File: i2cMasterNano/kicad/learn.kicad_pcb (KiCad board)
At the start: 2 copper layers, 27 parts, among them J1 Conn_01x04_Male, J10 Conn_01x01, J2 Conn_01x04_Male, J3 Conn_01x04_Male, J4 Conn_01x04_Male, J5 Conn_01x04_Male, J6 Conn_01x04_Male, J7 Conn_01x04_Male, J8 Conn_01x04_Male, J9 Conn_01x01, SW1 SW_DIP_x03, U1 LM7805_TO220, U2 Arduino_Nano_R3

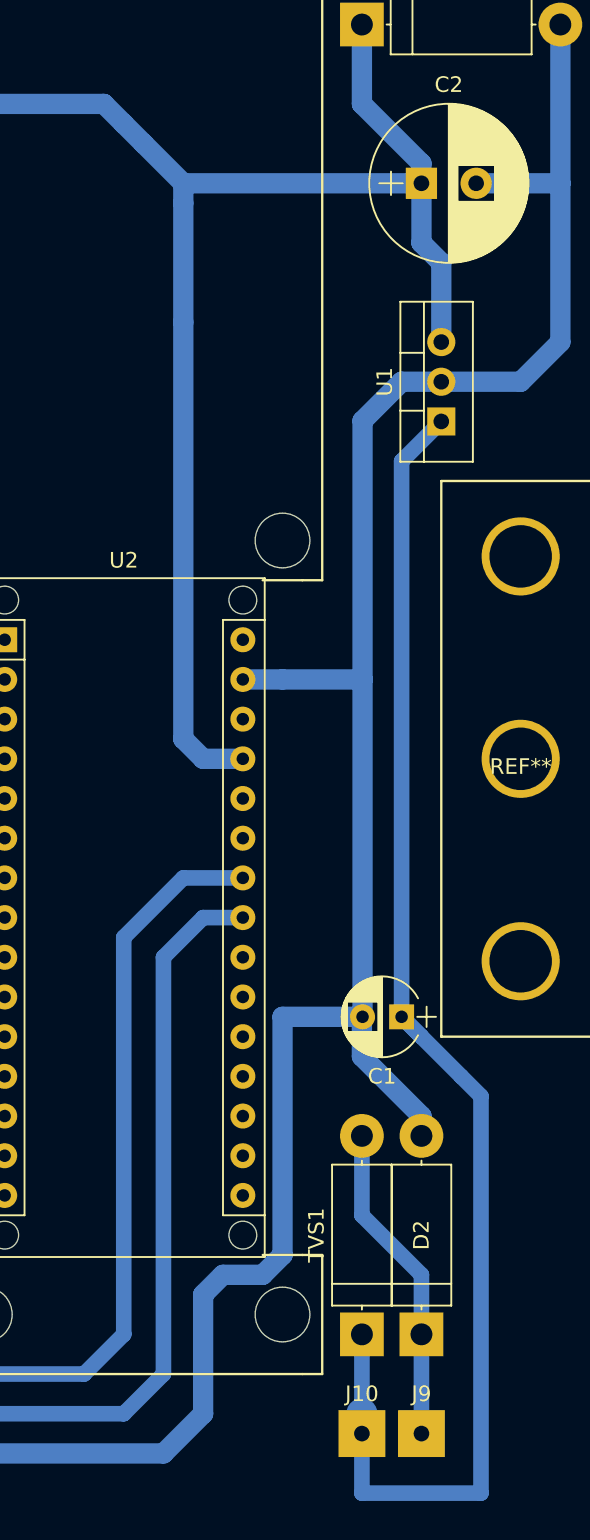
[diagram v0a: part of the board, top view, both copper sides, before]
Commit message: ...
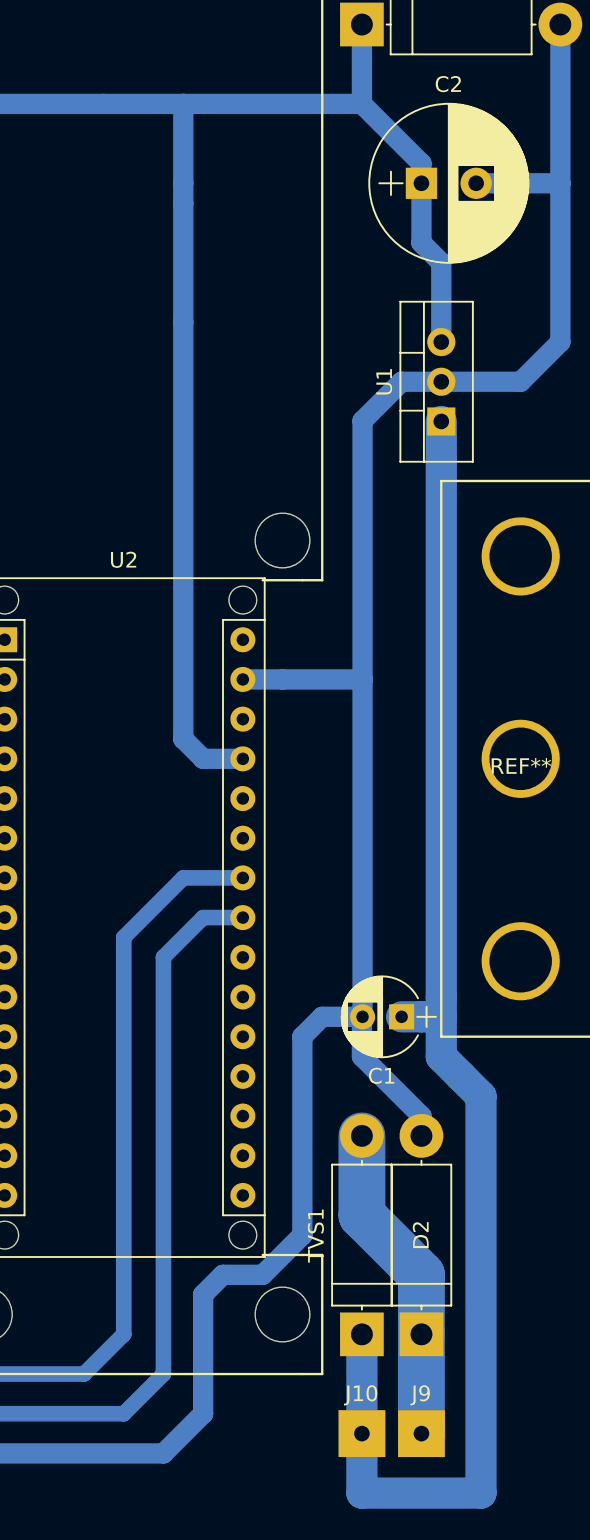
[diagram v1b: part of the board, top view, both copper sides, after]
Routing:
- net GND: track 265.1 -> 263.6 mm
- net Net-(C1-Pad1): track 92.6 -> 91.2 mm
- net +5V: track 230.1 -> 229.3 mm
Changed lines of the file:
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@@
     (links 63)
     (no_connects 1)
-    (area 129.064999 65.765 213.460001 165.200001)
+    (area 129.064999 65.765 207.485001 165.230002)
     (thickness 1.6)
     (drawings 6)
-    (tracks 163)
+    (tracks 165)
     (zones 0)
     (modules 27)
@@
   )
   (setup
-    (last_trace_width 1)
+    (last_trace_width 2)
     (user_trace_width 1)
     (user_trace_width 2)
@@
   (gr_line (start 207.01 66.04) (end 207.01 111.76) (angle 90) (layer Margin) (width 0.2))
   (gr_line (start 129.54 163.83) (end 129.54 66.04) (angle 90) (layer Margin) (width 0.2))
+  (segment (start 187.96 134.62) (end 189.23 133.35) (width 1.3) (layer B.Cu) (net 1))
   (segment (start 199.08 80.01) (end 204.47 80.01) (width 1.3) (layer B.Cu) (net 1))
   (segment (start 196.85 92.71) (end 201.93 92.71) (width 1.3) (layer B.Cu) (net 1))
@@
   (segment (start 204.47 80.01) (end 204.47 69.85) (width 1.3) (layer B.Cu) (net 1))
   (segment (start 201.93 92.71) (end 204.47 90.17) (width 1.3) (layer B.Cu) (net 1))
-  (segment (start 191.81 133.35) (end 186.69 133.35) (width 1.3) (layer B.Cu) (net 1))
+  (segment (start 191.81 133.35) (end 189.23 133.35) (width 1.3) (layer B.Cu) (net 1))
   (segment (start 186.69 111.76) (end 191.81 111.76) (width 1.3) (layer B.Cu) (net 1))
   (segment (start 191.81 111.76) (end 191.77 111.76) (width 1.3) (layer B.Cu) (net 1))
@@
   (segment (start 161.29 161.29) (end 162.56 161.29) (width 1.3) (layer B.Cu) (net 1))
   (segment (start 157.48 161.29) (end 154.94 161.29) (width 1.3) (layer B.Cu) (net 1) (status 10))
-  (segment (start 186.69 133.35) (end 186.69 148.59) (width 1.3) (layer B.Cu) (net 1))
-  (segment (start 186.69 148.59) (end 185.42 149.86) (width 1.3) (layer B.Cu) (net 1))
+  (segment (start 187.96 134.62) (end 187.96 147.32) (width 1.3) (layer B.Cu) (net 1))
+  (segment (start 187.96 147.32) (end 185.42 149.86) (width 1.3) (layer B.Cu) (net 1))
   (segment (start 185.42 149.86) (end 182.88 149.86) (width 1.3) (layer B.Cu) (net 1))
   (segment (start 182.88 149.86) (end 181.61 151.13) (width 1.3) (layer B.Cu) (net 1))
@@
   (segment (start 163.83 115.57) (end 165.1 116.84) (width 1.3) (layer B.Cu) (net 1))
   (segment (start 184.15 111.76) (end 186.69 111.76) (width 1.3) (layer B.Cu) (net 1) (status 10))
-  (segment (start 175.26 74.93) (end 176.53 76.2) (width 1.3) (layer B.Cu) (net 2))
-  (segment (start 177.8 77.47) (end 180.34 80.01) (width 1.3) (layer B.Cu) (net 2))
-  (segment (start 176.53 76.2) (end 177.8 77.47) (width 1.3) (layer B.Cu) (net 2))
-  (segment (start 195.58 80.01) (end 180.34 80.01) (width 1.3) (layer B.Cu) (net 2))
+  (segment (start 180.34 80.01) (end 180.34 74.93) (width 1.3) (layer B.Cu) (net 2))
+  (segment (start 175.26 74.93) (end 180.34 74.93) (width 1.3) (layer B.Cu) (net 2))
+  (segment (start 180.34 74.93) (end 191.77 74.93) (width 1.3) (layer B.Cu) (net 2))
   (segment (start 195.58 80.01) (end 195.58 78.74) (width 1.3) (layer B.Cu) (net 2))
   (segment (start 195.58 78.74) (end 191.77 74.93) (width 1.3) (layer B.Cu) (net 2))
@@
   (segment (start 176.53 128.27) (end 176.53 153.67) (width 1) (layer B.Cu) (net 4))
   (segment (start 180.34 124.46) (end 176.53 128.27) (width 1) (layer B.Cu) (net 4))
-  (segment (start 196.85 95.25) (end 194.31 97.79) (width 1) (layer B.Cu) (net 24))
-  (segment (start 194.31 97.79) (end 194.31 133.35) (width 1) (layer B.Cu) (net 24))
-  (segment (start 194.31 133.35) (end 195.58 134.62) (width 1) (layer B.Cu) (net 24))
-  (segment (start 198.12 137.16) (end 199.39 138.43) (width 1) (layer B.Cu) (net 24))
-  (segment (start 191.77 160.02) (end 191.77 163.83) (width 1) (layer B.Cu) (net 24))
-  (segment (start 191.77 163.83) (end 199.39 163.83) (width 1) (layer B.Cu) (net 24))
-  (segment (start 199.39 163.83) (end 199.39 138.43) (width 1) (layer B.Cu) (net 24))
-  (segment (start 198.12 137.16) (end 195.58 134.62) (width 1) (layer B.Cu) (net 24))
-  (segment (start 195.58 134.62) (end 194.31 133.35) (width 1) (layer B.Cu) (net 24))
-  (segment (start 191.77 160.02) (end 191.77 153.67) (width 1) (layer B.Cu) (net 24))
+  (segment (start 196.85 135.89) (end 196.85 133.35) (width 2) (layer B.Cu) (net 24))
+  (segment (start 194.31 133.35) (end 195.58 133.35) (width 2) (layer B.Cu) (net 24))
+  (segment (start 195.58 133.35) (end 196.85 133.35) (width 2) (layer B.Cu) (net 24))
+  (segment (start 196.85 95.25) (end 196.85 97.79) (width 2) (layer B.Cu) (net 24))
+  (segment (start 196.85 97.79) (end 196.85 132.08) (width 2) (layer B.Cu) (net 24))
+  (segment (start 196.85 132.08) (end 196.85 133.35) (width 2) (layer B.Cu) (net 24))
+  (segment (start 198.12 137.16) (end 199.39 138.43) (width 2) (layer B.Cu) (net 24))
+  (segment (start 191.77 160.02) (end 191.77 163.83) (width 2) (layer B.Cu) (net 24))
+  (segment (start 191.77 163.83) (end 199.39 163.83) (width 2) (layer B.Cu) (net 24))
+  (segment (start 199.39 163.83) (end 199.39 138.43) (width 2) (layer B.Cu) (net 24))
+  (segment (start 198.12 137.16) (end 196.85 135.89) (width 2) (layer B.Cu) (net 24))
+  (segment (start 191.77 160.02) (end 191.77 153.67) (width 2) (layer B.Cu) (net 24))
   (segment (start 191.77 160.02) (end 191.77 158.75) (width 2) (layer B.Cu) (net 24) (status 30))
   (segment (start 196.85 95.25) (end 196.85 95.25) (width 2) (layer B.Cu) (net 24) (status 30))
@@
   (segment (start 168.91 132.08) (end 166.37 132.08) (width 0.8) (layer B.Cu) (net 35))
   (segment (start 166.37 132.08) (end 163.83 135.89) (width 0.8) (layer B.Cu) (net 35) (status 20))
-  (segment (start 195.58 153.67) (end 195.58 149.86) (width 1) (layer B.Cu) (net 36))
-  (segment (start 191.77 146.05) (end 191.77 140.97) (width 1) (layer B.Cu) (net 36))
-  (segment (start 195.58 149.86) (end 191.77 146.05) (width 1) (layer B.Cu) (net 36))
-  (segment (start 195.58 160.02) (end 195.58 153.67) (width 1) (layer B.Cu) (net 36))
+  (segment (start 195.58 153.67) (end 195.58 149.86) (width 3) (layer B.Cu) (net 36))
+  (segment (start 191.77 146.05) (end 191.77 140.97) (width 3) (layer B.Cu) (net 36))
+  (segment (start 195.58 149.86) (end 191.77 146.05) (width 3) (layer B.Cu) (net 36))
+  (segment (start 195.58 160.02) (end 195.58 153.67) (width 3) (layer B.Cu) (net 36))
 )
